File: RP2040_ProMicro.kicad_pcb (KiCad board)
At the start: 2 copper layers, 23 x 51 mm, 50 parts, among them J1 HRO_TYPE-C-31-M-14, J2 Conn_01x16, J3 Battery, J6 Conn_01x12, Q1 SI2301A, SW1 SW_Push, SW2 SW_Push, U1 USBLC6-2SC6, U2 SOT23-5 200mA 3.3V, U3 TP4054, U4 RP2040, U5 W25Q128JVS, Y1 Crystal_GND23

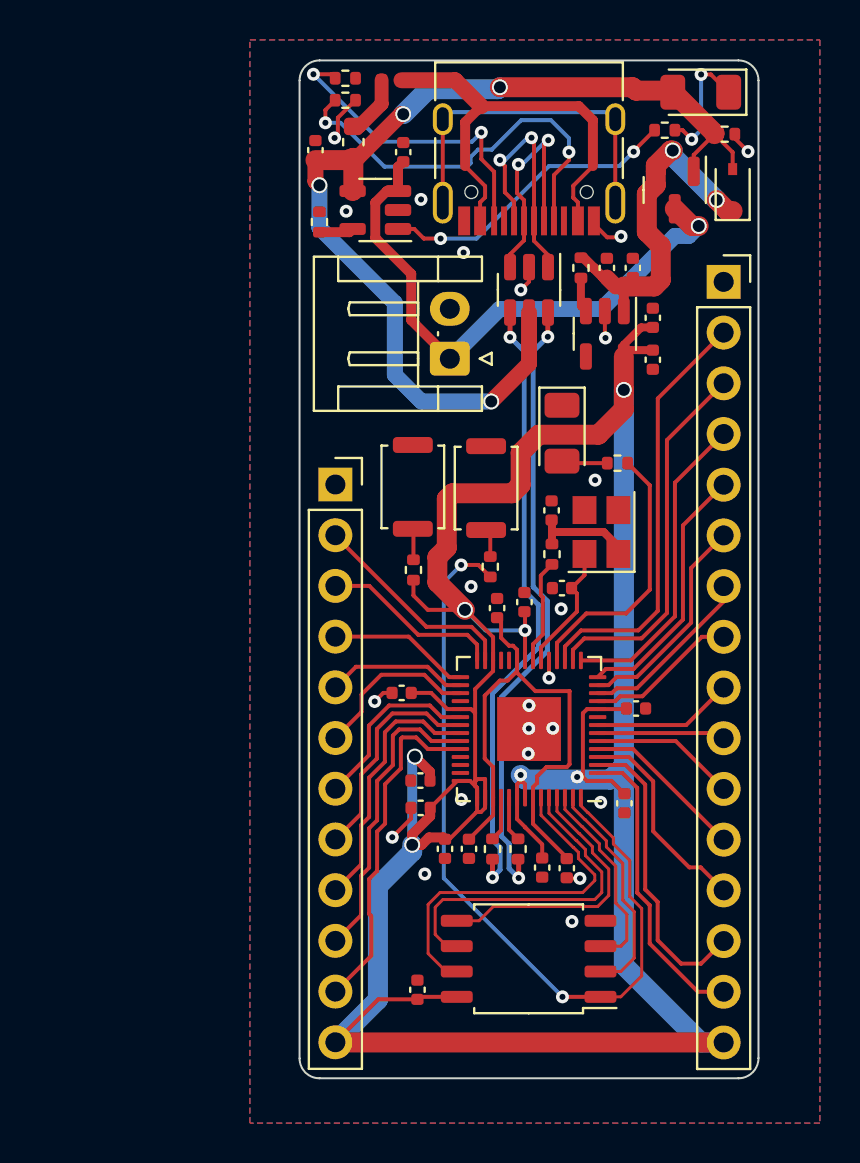
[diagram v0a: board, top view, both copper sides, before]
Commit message: Routing in progress
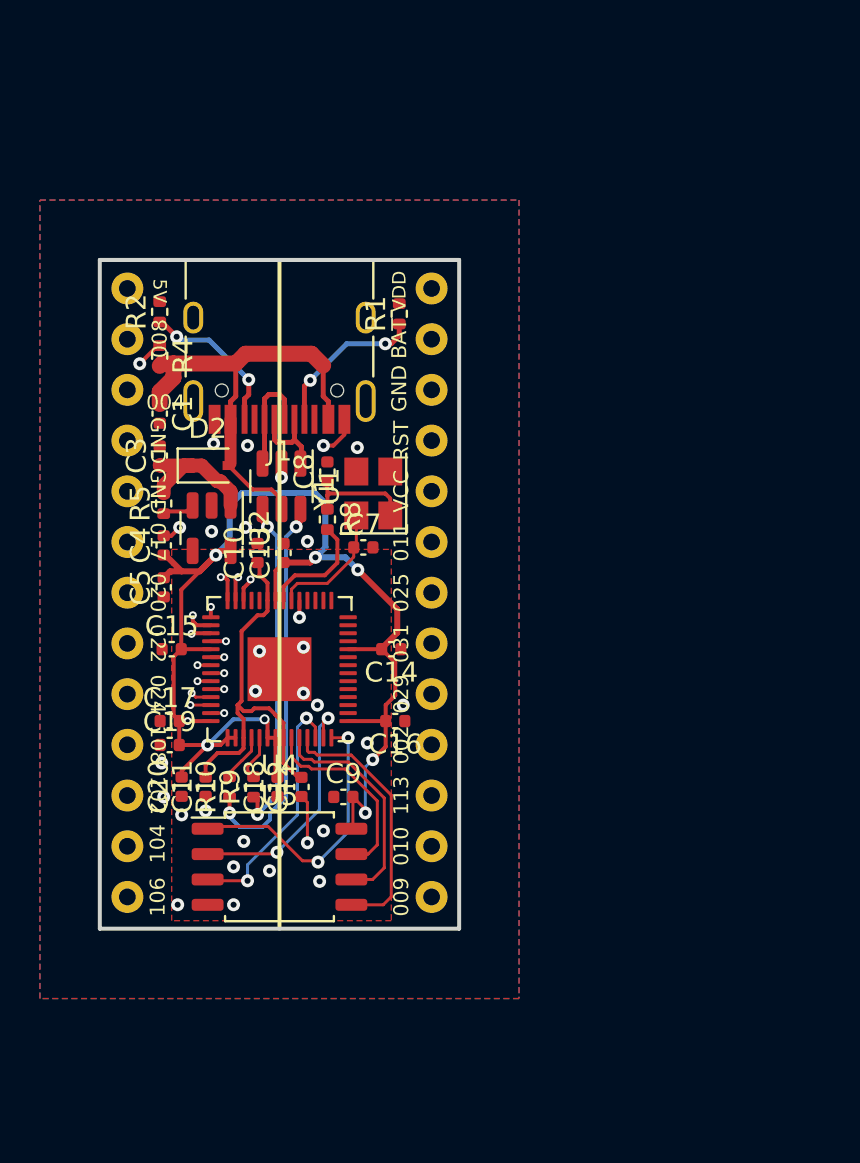
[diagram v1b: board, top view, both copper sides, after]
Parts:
- removed C2, C6: 10uF, Capacitor_SMD:C_0402_1005Metric
- removed D1, D3: LED, LED_SMD:LED_1206_3216Metric
- removed F1: 750 mA, Fuse:Fuse_0603_1608Metric
- removed J3: Battery, Connector_JST:JST_EH_S2B-EH_1x02_P2.50mm_Horizontal
- removed J6: Conn_01x12, Connector_PinSocket_2.54mm:PinSocket_1x12_P2.54mm_Vertical
- removed L1: BLM15PX121SN1D, Inductor_SMD:L_0402_1005Metric
- removed Q1: SI2301A, Package_TO_SOT_SMD:SOT-23
- removed R11, R12, R7: 1k, Resistor_SMD:R_0402_1005Metric
- removed R3: 470, Resistor_SMD:R_0402_1005Metric
- removed R6: 2k, Resistor_SMD:R_0402_1005Metric
- removed SW1, SW2: SW_Push, Button_Switch_SMD:SW_Push_SPST_NO_Alps_SKRK
- removed U3: TP4054, Package_TO_SOT_SMD:SOT-23-5
- J2: value Conn_01x16 -> Conn_01x26; footprint Connector_PinSocket_2.54mm:PinSocket_1x16_P2.54mm_Vertical -> mikotofootprints:mikoto-pins
- R10, R9: value 27 -> 27R
- moved R4 30.4 mm to (153.0, 34.8), turned to -90 degrees
- moved D2 29.7 mm to (155.4, 40.3), turned to 0 degrees
- moved J2 27.9 mm to (159.0, 47.9)
- moved C4 27.0 mm to (153.2, 44.3)
- moved C5 27.0 mm to (153.2, 46.4)
- moved C3 25.5 mm to (153.0, 39.8)
- moved R5 24.0 mm to (153.2, 42.2)
- moved U2 22.0 mm to (155.6, 43.4)
- moved C19 19.6 mm to (153.5, 54.3), turned to 0 degrees
- moved C11 18.5 mm to (155.3, 56.4)
- moved J1 16.0 mm to (159.0, 33.9)
- moved U1 15.8 mm to (159.1, 41.3)
- moved C1 15.3 mm to (153.0, 37.7)
- moved R2 14.9 mm to (153.0, 32.6), turned to 90 degrees
- moved C14 14.0 mm to (164.6, 49.5), turned to 180 degrees
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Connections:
- C1 pad 1: GND -> +5V
- C1 pad 2: +5V -> GND
- J1 pad A4: VBUS -> +5V
- J1 pad A9: VBUS -> +5V
- J1 pad B4: VBUS -> +5V
- J1 pad B9: VBUS -> +5V
- J2 pad 1: GND -> +5V
- J2 pad 10: /GPIO5 -> unconnected-(J2-Pad10)
- J2 pad 11: /GPIO4 -> unconnected-(J2-Pad11)
- J2 pad 12: /GPIO3 -> unconnected-(J2-Pad12)
- J2 pad 13: /GPIO2 -> unconnected-(J2-Pad13)
- J2 pad 14: /GPIO1 -> unconnected-(J2-Pad14)
- J2 pad 15: /GPIO0 -> unconnected-(J2-Pad15)
- J2 pad 16: +3V3 -> unconnected-(J2-Pad16)
- J2 pad 2: /GPIO14 -> unconnected-(J2-Pad2)
- J2 pad 3: /GPIO13 -> unconnected-(J2-Pad3)
- J2 pad 4: /GPIO12 -> GND
- J2 pad 5: /GPIO11 -> GND
- J2 pad 6: /GPIO10 -> unconnected-(J2-Pad6)
- J2 pad 7: /GPIO9 -> unconnected-(J2-Pad7)
- J2 pad 8: /GPIO8 -> unconnected-(J2-Pad8)
- J2 pad 9: /GPIO6 -> unconnected-(J2-Pad9)
- U1 pad 1: D+ -> D-
- U1 pad 3: D- -> D+
- U1 pad 4: USB_D- -> USB_D+
- U1 pad 6: USB_D+ -> USB_D-
- U4 pad 26: +3V3 -> /RESET
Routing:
- net +3V3: track 159.9 -> 69.4 mm, vias 7 -> 8
- net +BATT: track 29.1 -> 0.00 mm, vias 1 -> 0
- net +5V: track 51.6 -> 23.0 mm, vias 4 -> 0
- net QSPI_SS: track 40.8 -> 14.1 mm
- net VBUS: track 22.6 -> 0.00 mm
- net /GPIO14: track 21.4 -> 0.00 mm
- net /GPIO13: track 18.7 -> 0.00 mm
- net unconnected-(J1-PadS1): track 17.3 -> 0.00 mm
- net /GPIO26: track 17.4 -> 0.67 mm, vias 0 -> 1
- net /GPIO12: track 15.8 -> 0.00 mm
- net Net-(R7-Pad1): track 15.3 -> 0.00 mm, vias 2 -> 0
- net /GPIO1: track 15.1 -> 0.00 mm
- net /GPIO0: track 15.1 -> 0.00 mm
- net /GPIO25: track 15.2 -> 0.67 mm, vias 0 -> 1
- net USB_D+: track 31.2 -> 16.8 mm
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- added copper zone on F.Cu, net +3V3
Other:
- board size 23 x 51 mm -> 18 x 33.5 mm
